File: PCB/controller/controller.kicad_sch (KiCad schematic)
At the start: 27 parts, among them U1 RP2040_Pro_Micro, X1 Switch, Y1 Switch

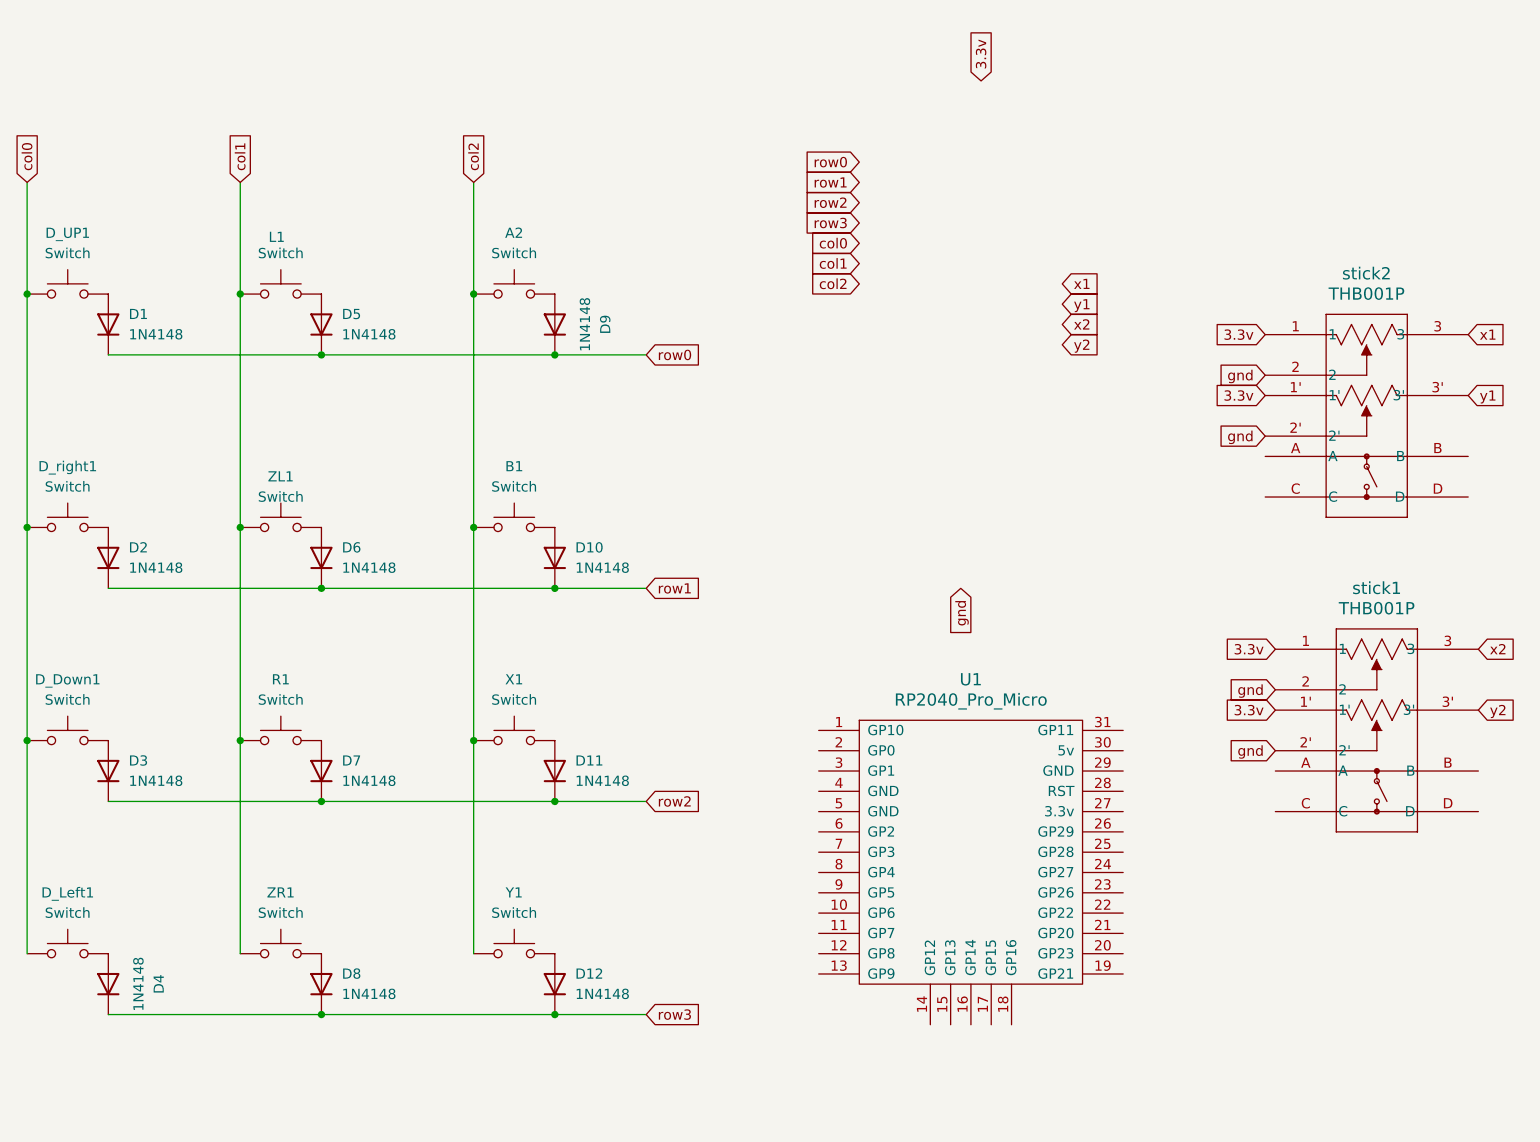
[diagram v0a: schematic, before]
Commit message: adding stuff
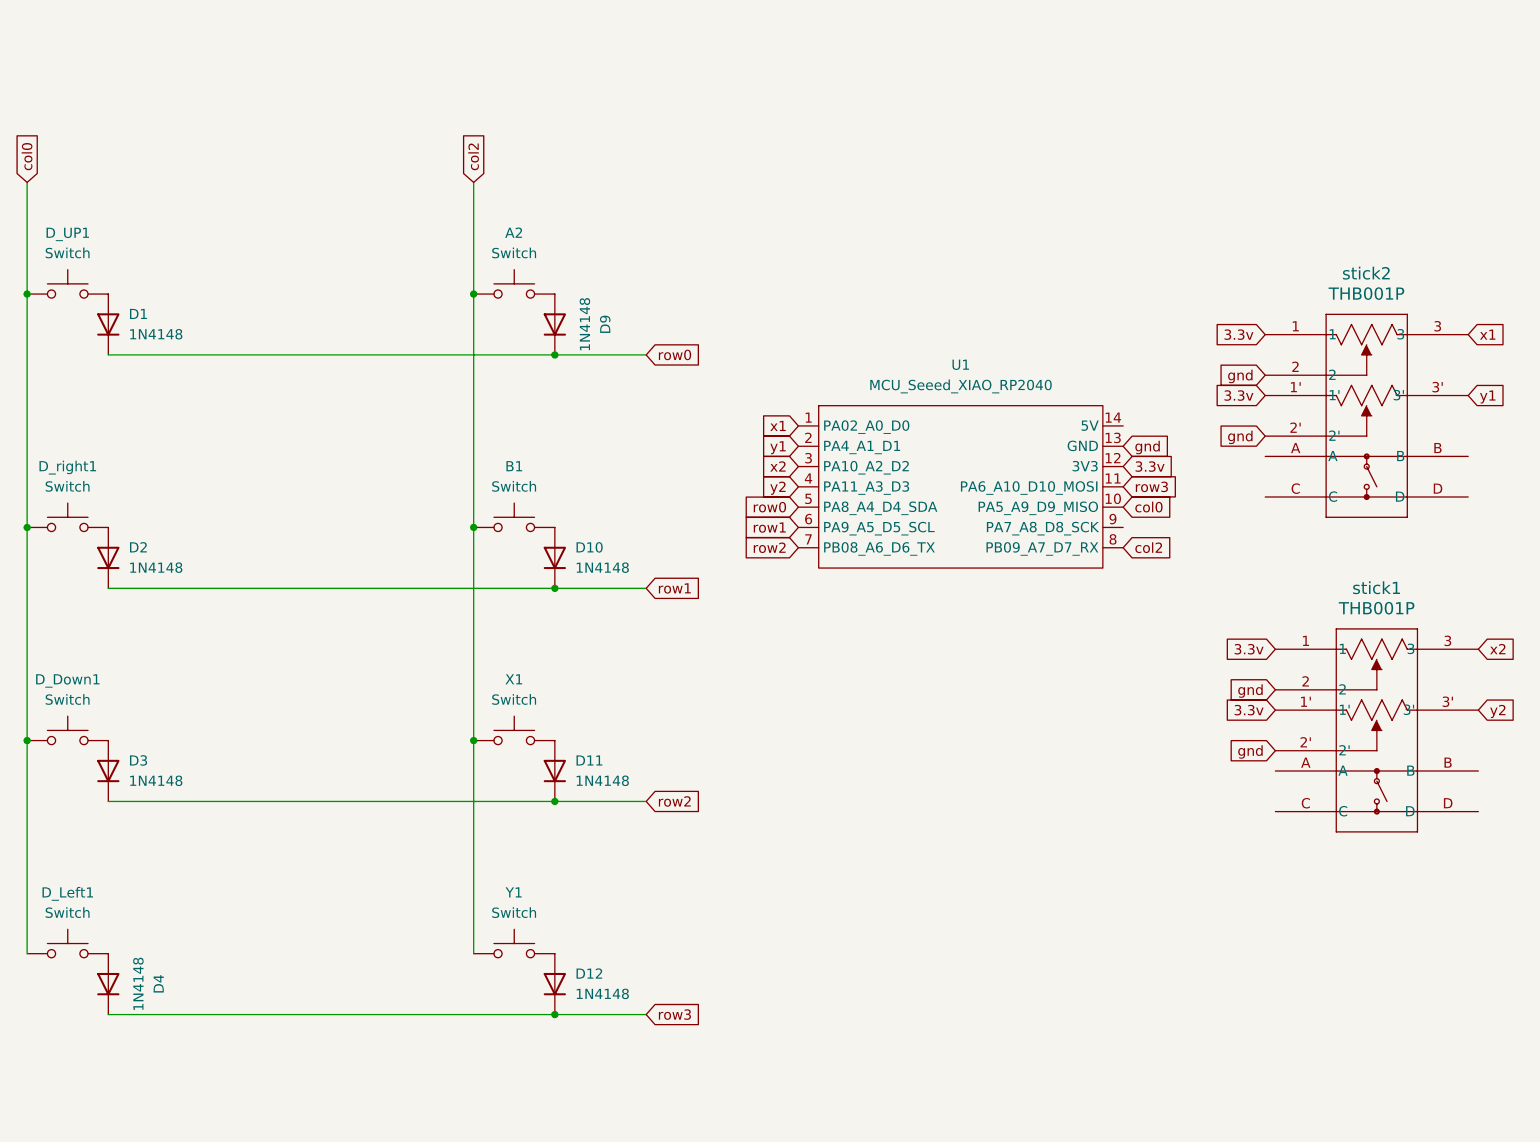
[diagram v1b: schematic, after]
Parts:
- removed D5, D6, D7, D8: 1N4148, Diode_THT:D_DO-35_SOD27_P7.62mm_Horizontal, symbol Diode:1N4148
- removed L1, R1, ZL1, ZR1: Switch, Button_Switch_SMD:SW_Push_1P1T_NO_CK_KSC6xxJ, symbol ScottoKeebs:Placeholder_Switch
- removed U1: RP2040_Pro_Micro, ScottoKeebs_MCU:RP2040_Pro_Micro, symbol ScottoKeebs:MCU_RP2040_Pro_Micro
- added U1: MCU_Seeed_XIAO_RP2040, ScottoKeebs_MCU:Seeed_XIAO_RP2040, symbol ScottoKeebs:MCU_Seeed_XIAO_RP2040
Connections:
- net 3.3v: now also U1.12 (3V3)
- net col0: now also U1.10 (PA5_A9_D9_MISO)
- net col2: now also U1.8 (PB09_A7_D7_RX)
- net gnd: now also U1.13 (GND)
- net row0: now also U1.5 (PA8_A4_D4_SDA)
- net row1: now also U1.6 (PA9_A5_D5_SCL)
- net row2: now also U1.7 (PB08_A6_D6_TX)
- net row3: now also U1.11 (PA6_A10_D10_MOSI)
- net x1: now also U1.1 (PA02_A0_D0)
- net x2: now also U1.3 (PA10_A2_D2)
- net y1: now also U1.2 (PA4_A1_D1)
- net y2: now also U1.4 (PA11_A3_D3)

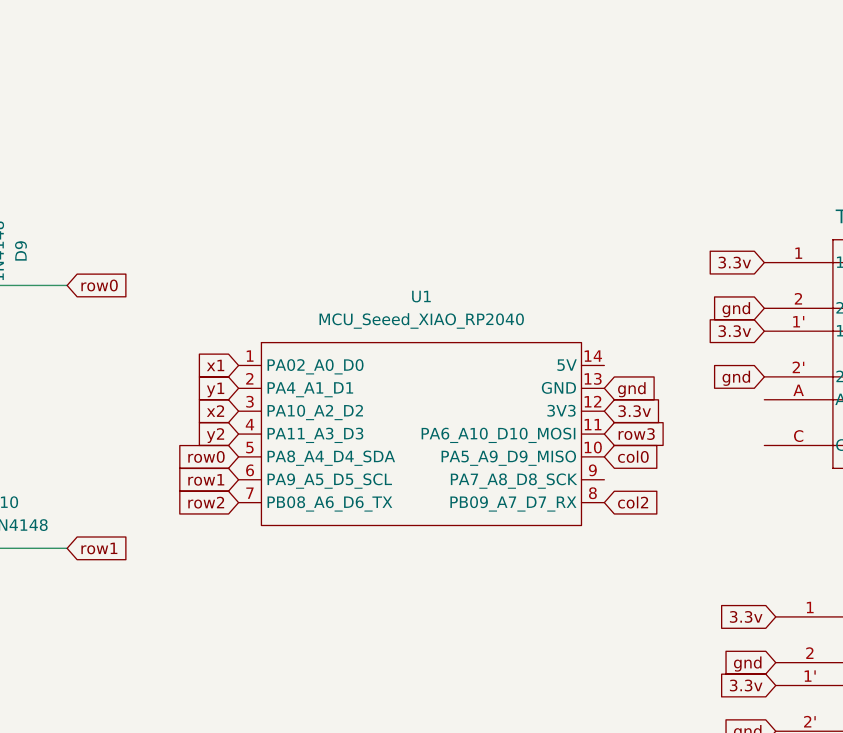
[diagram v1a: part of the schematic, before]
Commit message: finishing
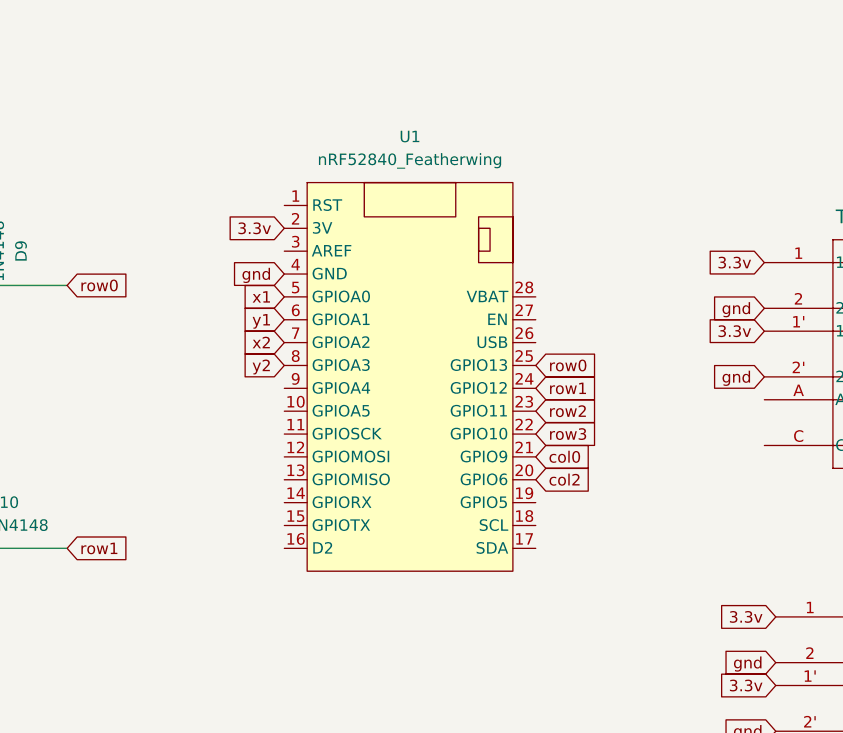
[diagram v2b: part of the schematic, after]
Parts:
- removed U1: MCU_Seeed_XIAO_RP2040, ScottoKeebs_MCU:Seeed_XIAO_RP2040, symbol ScottoKeebs:MCU_Seeed_XIAO_RP2040
- added U1: nRF52840_Featherwing, Module:Adafruit_Feather, symbol dumb:nRF52840_Featherwing
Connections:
- net 3.3v: now also U1.2 (3V)
- net col0: now also U1.21 (GPIO9)
- net col2: now also U1.20 (GPIO6)
- net gnd: now also U1.4 (GND)
- net row0: now also U1.25 (GPIO13)
- net row1: now also U1.24 (GPIO12)
- net row2: now also U1.23 (GPIO11)
- net row3: now also U1.22 (GPIO10)
- net x1: now also U1.5 (GPIOA0)
- net x2: now also U1.7 (GPIOA2)
- net y1: now also U1.6 (GPIOA1)
- net y2: now also U1.8 (GPIOA3)

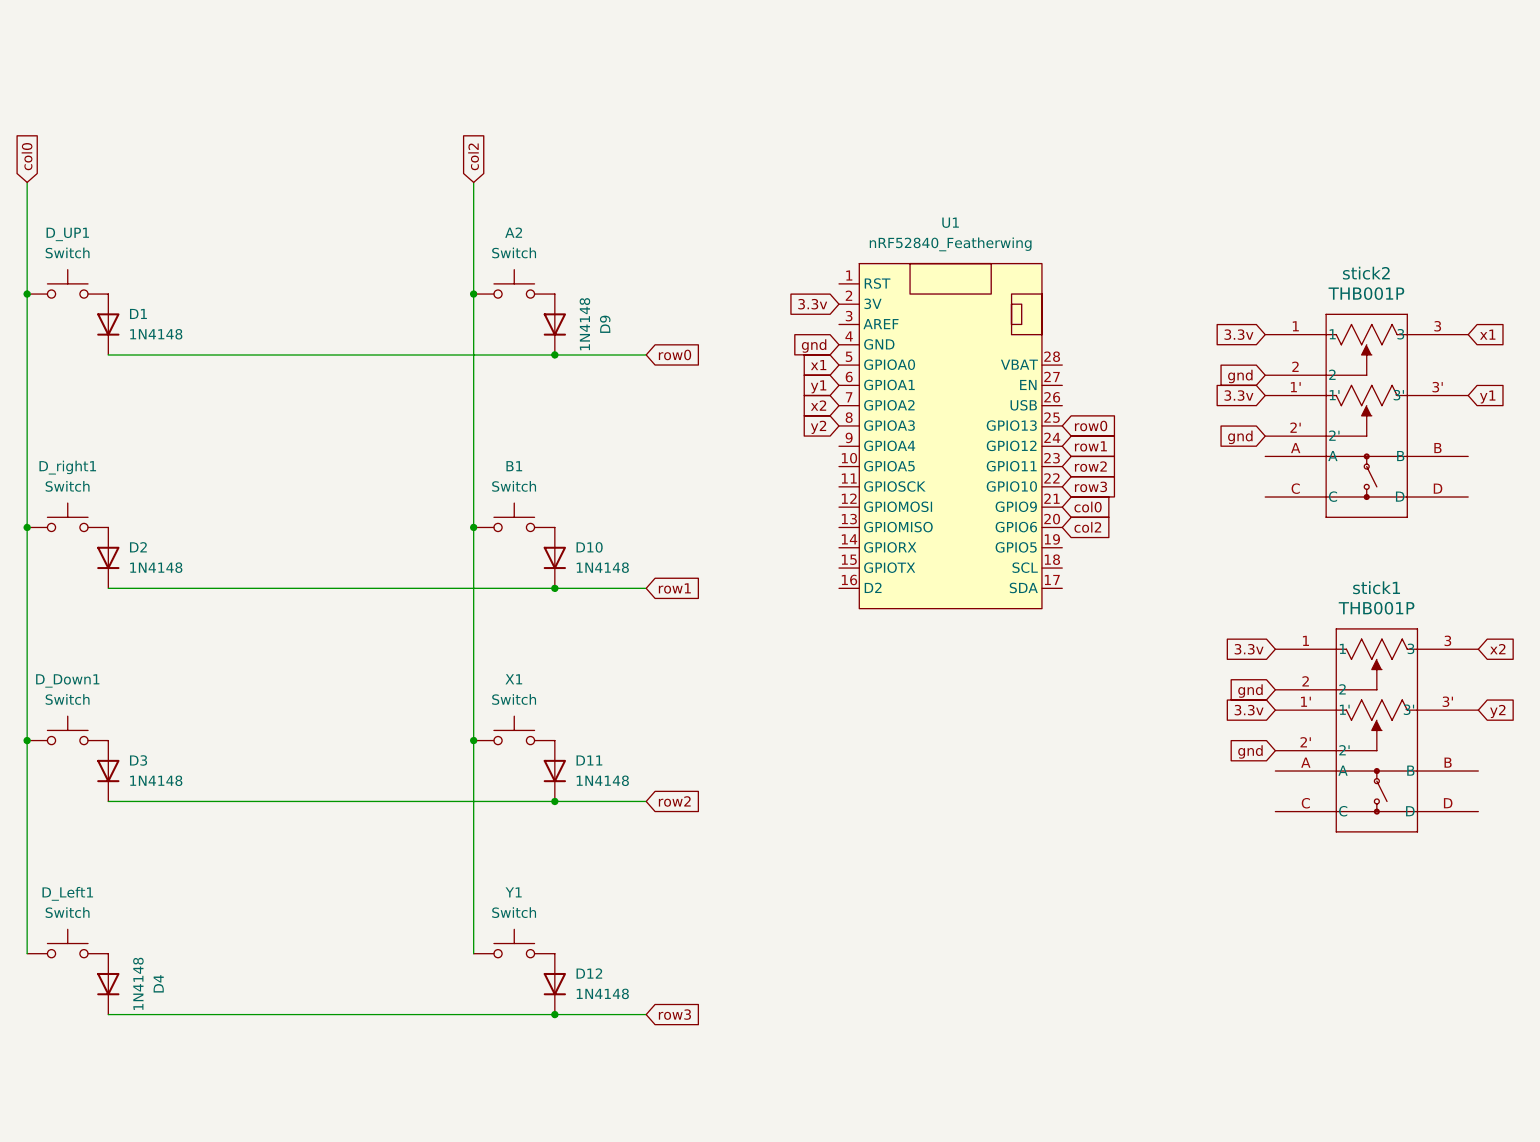
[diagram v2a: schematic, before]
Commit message: firmwere
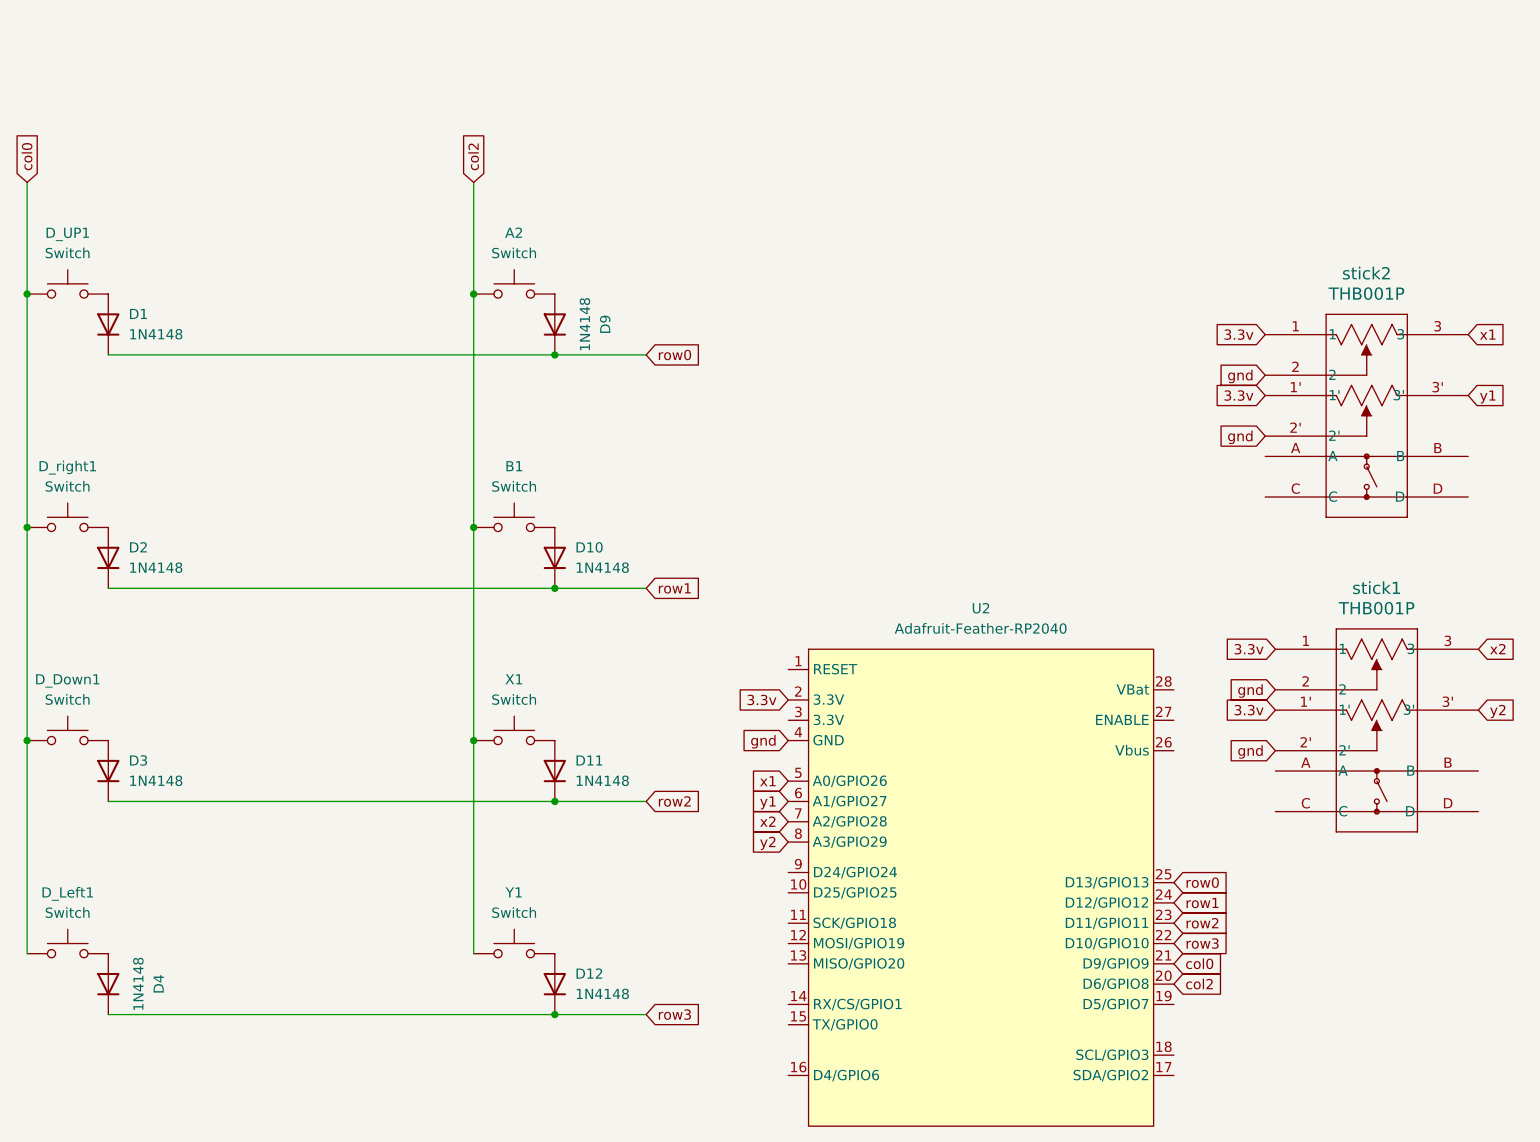
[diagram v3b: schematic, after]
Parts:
- removed U1: nRF52840_Featherwing, Module:Adafruit_Feather, symbol dumb:nRF52840_Featherwing
- added U2: Adafruit-Feather-RP2040, Module:Adafruit_Feather, symbol Adafruit-Feather-RP2040:Adafruit-Feather-RP2040
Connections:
- net 3.3v: now also U2.2 (3.3V)
- net col0: now also U2.21 (D9/GPIO9)
- net col2: now also U2.20 (D6/GPIO8)
- net gnd: now also U2.4 (GND)
- net row0: now also U2.25 (D13/GPIO13)
- net row1: now also U2.24 (D12/GPIO12)
- net row2: now also U2.23 (D11/GPIO11)
- net row3: now also U2.22 (D10/GPIO10)
- net x1: now also U2.5 (A0/GPIO26)
- net x2: now also U2.7 (A2/GPIO28)
- net y1: now also U2.6 (A1/GPIO27)
- net y2: now also U2.8 (A3/GPIO29)
